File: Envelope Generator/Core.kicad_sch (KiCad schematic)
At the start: 34 parts, among them J201 AudioJack2_SwitchT, Q201 BC547, Q202 BC547, Q203 BC547, SW201 SW_SPST, SW202 SW_SPDT, U101 TL072, U102 TL072, U201 ICM7555xP

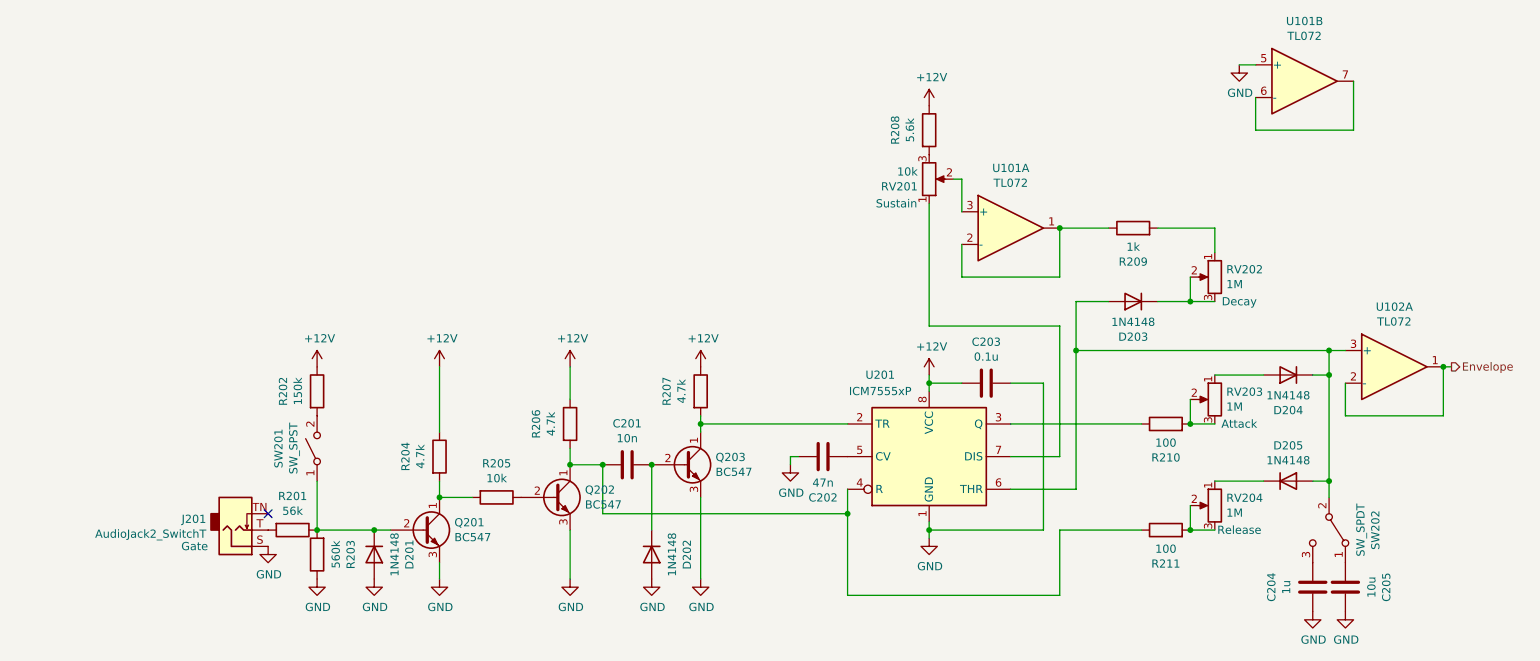
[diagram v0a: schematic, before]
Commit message: New modules, small updates
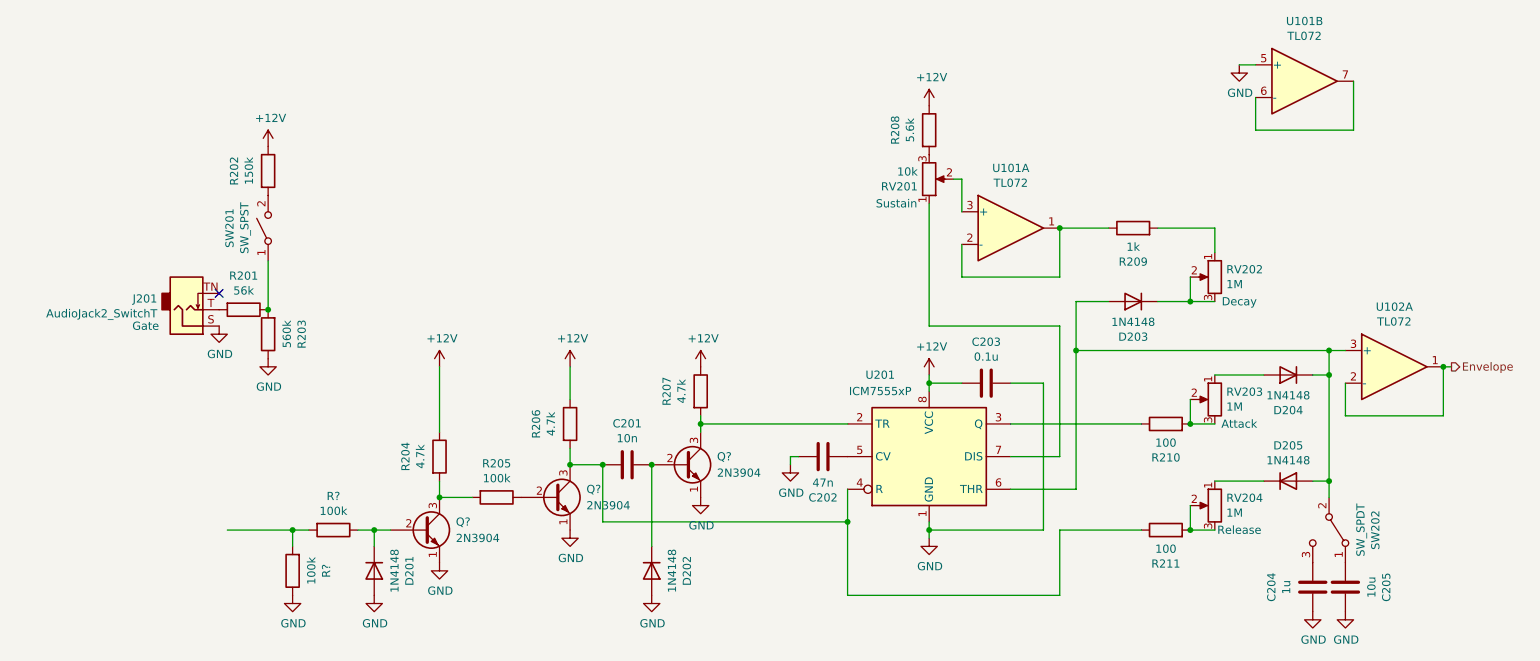
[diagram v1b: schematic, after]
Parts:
- removed Q201, Q202, Q203: BC547, Package_TO_SOT_THT:TO-92_Inline, symbol Transistor_BJT:BC547
- added Q? (x3): 2N3904, Package_TO_SOT_THT:TO-92_Inline, symbol Transistor_BJT:2N3904
- added R? (x2): 100k, Resistor_THT:R_Axial_DIN0207_L6.3mm_D2.5mm_P7.62mm_Horizontal, symbol Device:R
- R205: value 10k -> 100k
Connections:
- net GND: now also Q?.1 (E), Q?.1 (E), Q?.1 (E), R?.1
- net at R207.2, U201.2 (TR): now also Q?.3 (C)
- net at C201.1, R206.2, R211.1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: now also Q?.3 (C)
- net at R204.2, R205.2: now also Q?.3 (C)
- net at R201.1, R203.2, SW201.1 (A): no longer D201.1 (K)
- net at R205.1: now also Q?.2 (B)
- net at C201.2, D202.1 (K): now also Q?.2 (B)
- new net: D201.1 (K), Q?.2 (B), R?.1
- new net: R?.2, R?.2
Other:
- moved on the sheet: D201, D202, J201, R201, R202, R203, SW201
